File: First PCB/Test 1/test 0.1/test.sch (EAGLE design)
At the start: 9 parts, among them SW2 B3U-1000P

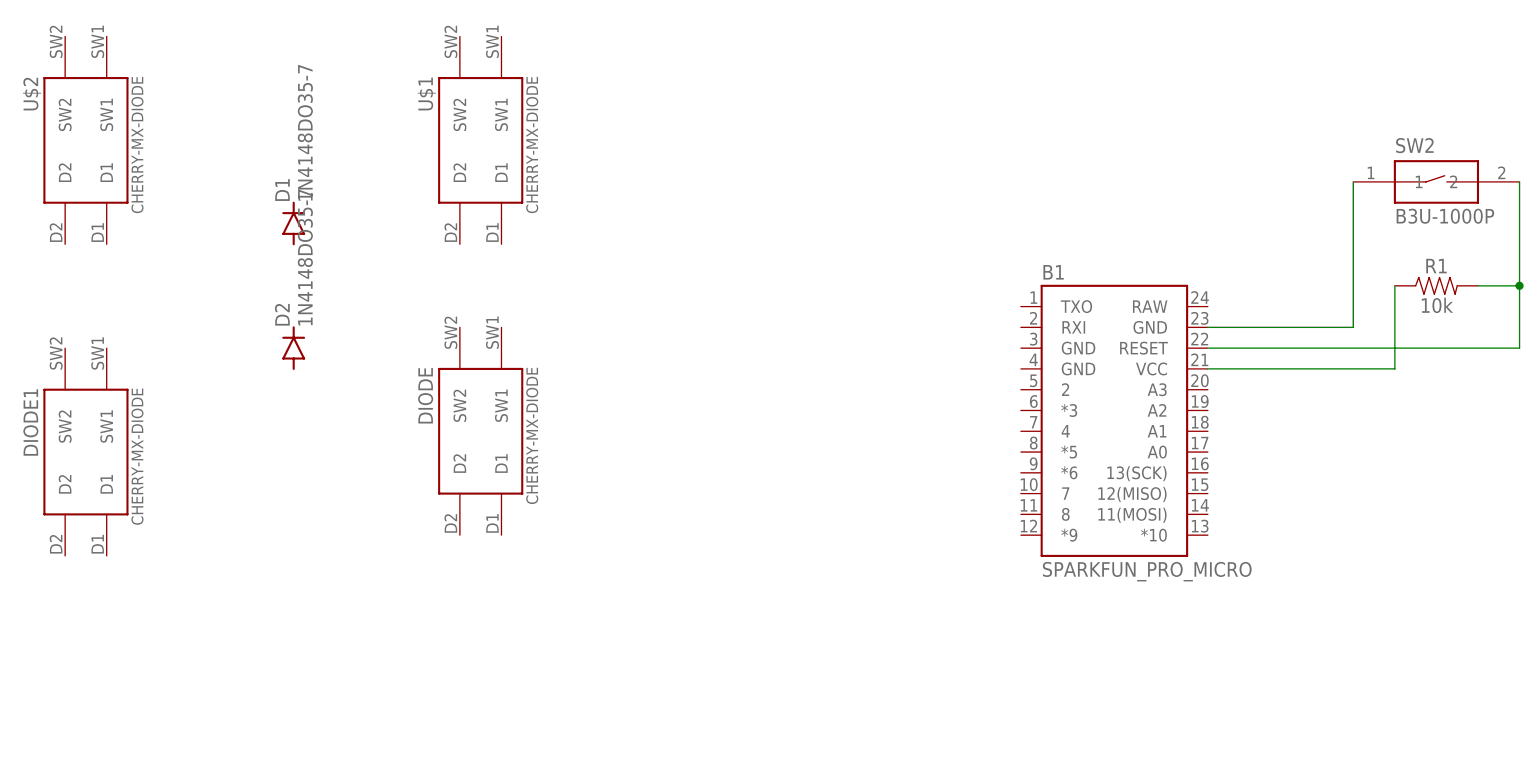
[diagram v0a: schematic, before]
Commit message: finished board and submitted for review, https://geekhack.org/index.php?topic=102077.0
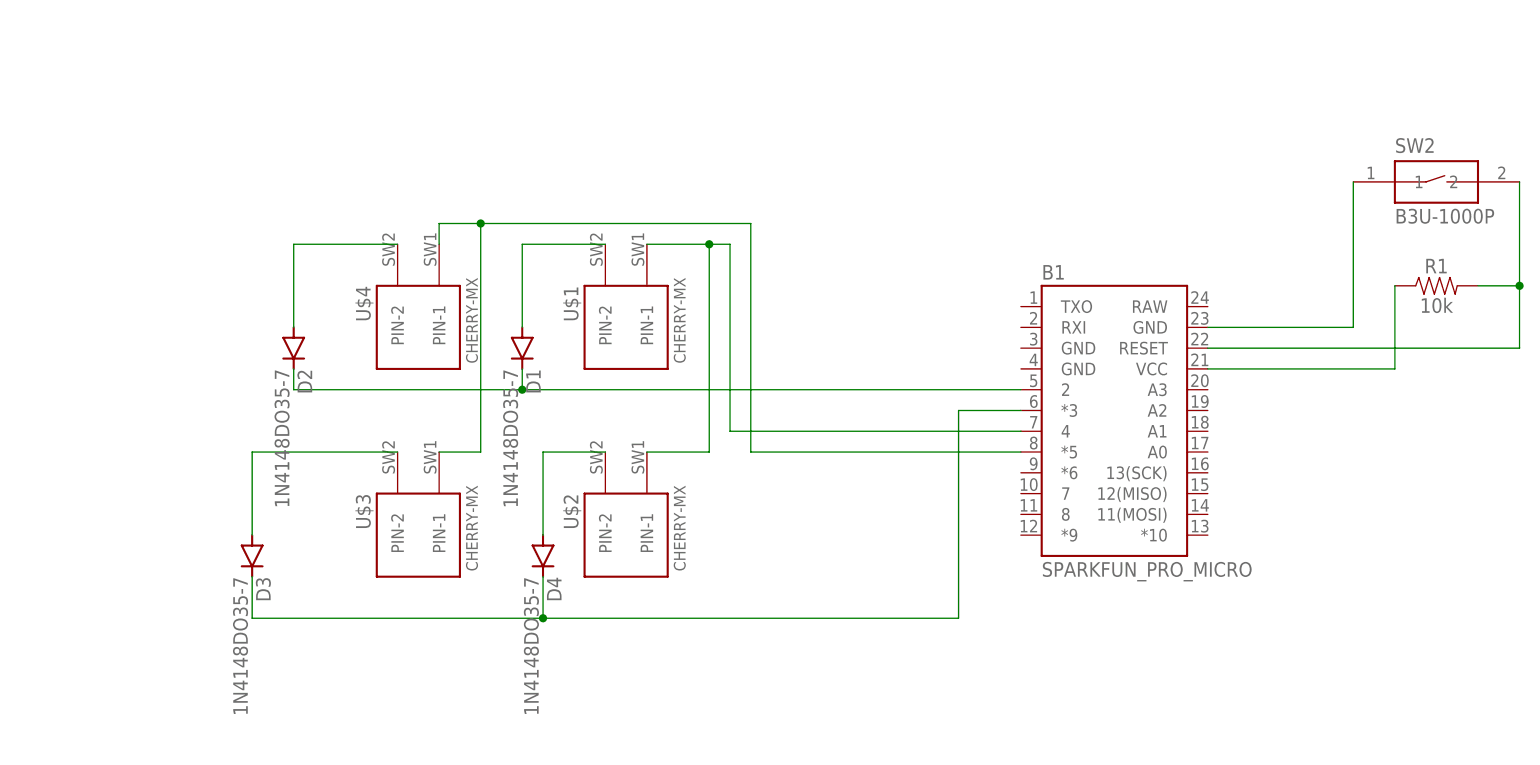
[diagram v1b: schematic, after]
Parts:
- removed DIODE, DIODE1: CHERRY-MX-DIODE, cherrymx:CHERRY-MX-DIODE
- added D3, D4: 1N4148DO35-7, diode:1N4148DO35-7
- added U$3, U$4: CHERRY-MX, cherrymx:CHERRY-MX
- U$1, U$2: value CHERRY-MX-DIODE -> CHERRY-MX; device cherrymx:CHERRY-MX-DIODE -> cherrymx:CHERRY-MX
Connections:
- new net N$10: D4.A, U$2.PIN-2
- new net N$12: D3.A, U$3.PIN-2
- new net N$4: B1.2, D1.C, D2.C
- new net N$5: D1.A, U$1.PIN-2
- new net N$6: B1.4, U$1.PIN-1, U$2.PIN-1
- new net N$7: B1.*3, D3.C, D4.C
- new net N$8: D2.A, U$4.PIN-2
- new net N$9: B1.*5, U$3.PIN-1, U$4.PIN-1
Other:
- moved on the sheet: D1, D2
